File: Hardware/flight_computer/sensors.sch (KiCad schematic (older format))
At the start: 16 parts, among them U10 CAM-M8Q-0, U11 BMI088, U12 LIS3MDLTR, U13 Barometer

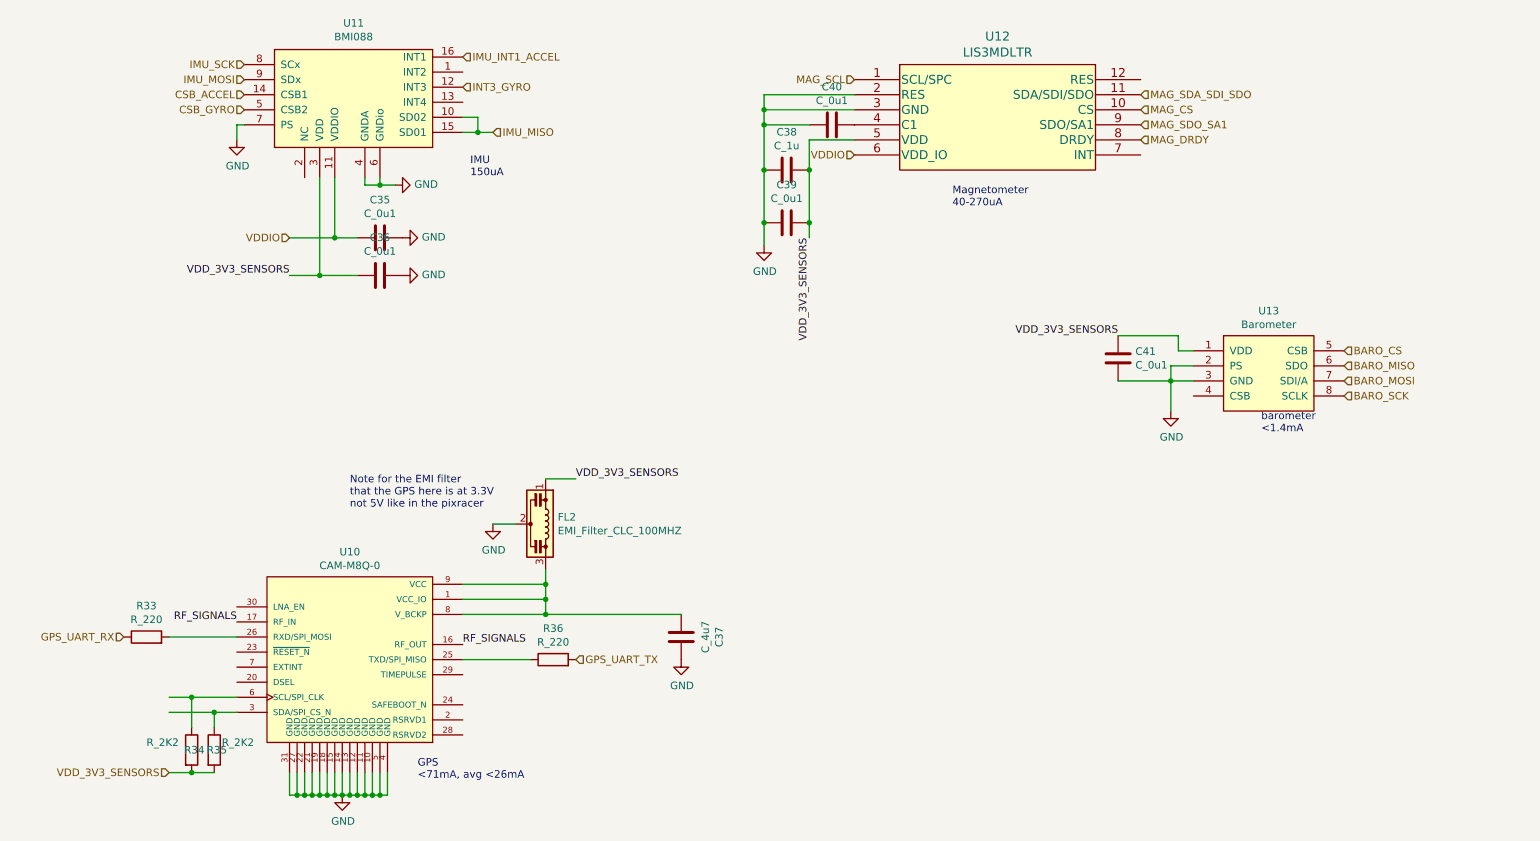
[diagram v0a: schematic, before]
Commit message: Finishes v1 connections
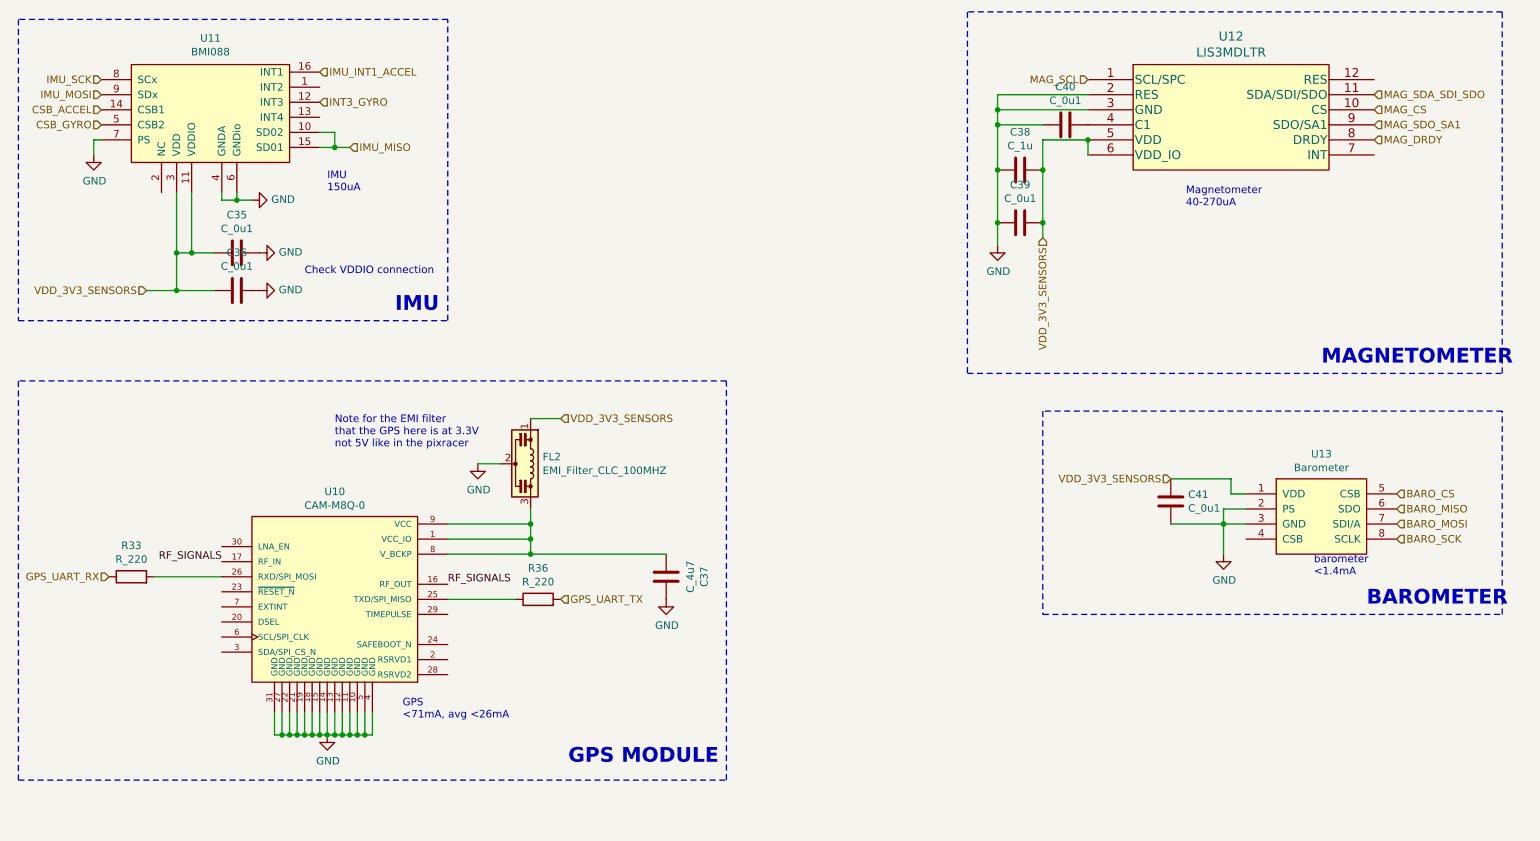
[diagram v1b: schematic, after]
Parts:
- removed R34, R35: R_2K2, Resistors_SMD:R_0805, symbol openDrone_parts:R_2K2
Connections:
- net VDDIO is gone; now on net VDD_3V3_SENSORS: C35.2, U11.11 (VDDIO), U12.6 (VDD_IO)
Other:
- note added: "BAROMETER"
- note added: "Check VDDIO connection"
- note added: "GPS MODULE"
- note added: "IMU"
- note added: "MAGNETOMETER"
- moved on the sheet: C35, C36, C37, C38, C39, C40, C41, FL2, R33, R36, U10, U11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
